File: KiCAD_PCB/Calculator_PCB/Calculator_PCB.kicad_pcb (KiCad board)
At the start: 2 copper layers, 132 x 78 mm, 110 parts, among them J1 USB_B_Micro, J2 5034801000, J3 5034801000, SW1 SW_SPST, SW10 SW_SPST, SW11 SW_SPST, SW12 SW_SPST, SW13 SW_SPST, SW14 SW_SPST, SW15 SW_SPST, SW16 SW_SPST, SW17 SW_SPST, SW18 SW_SPST, SW19 SW_SPST, SW2 SW_SPST, SW20 SW_SPST, SW21 SW_SPST, SW22 SW_SPST, SW23 SW_SPST, SW24 SW_SPST, SW25 SW_SPST, SW26 SW_SPST, SW27 SW_SPST, SW28 SW_SPST, SW29 SW_SPST, SW3 SW_SPST, SW30 SW_SPST, SW31 SW_SPST, SW32 SW_SPST, SW33 SW_SPST, SW34 SW_SPST, SW35 SW_SPST, SW36 SW_SPST, SW37 SW_SPST, SW38 SW_SPST, SW39 SW_SPST, SW4 SW_SPST, SW40 SW_SPST, SW5 SW_SPST, SW6 SW_SPST, SW7 SW_SPST, SW8 SW_SPST, SW9 SW_SPST, U1 W25Q128JVS, U2 RP2040, U3 NCP1117-3.3_SOT223, Y1 ABLS-12.000MHZ-B4-T

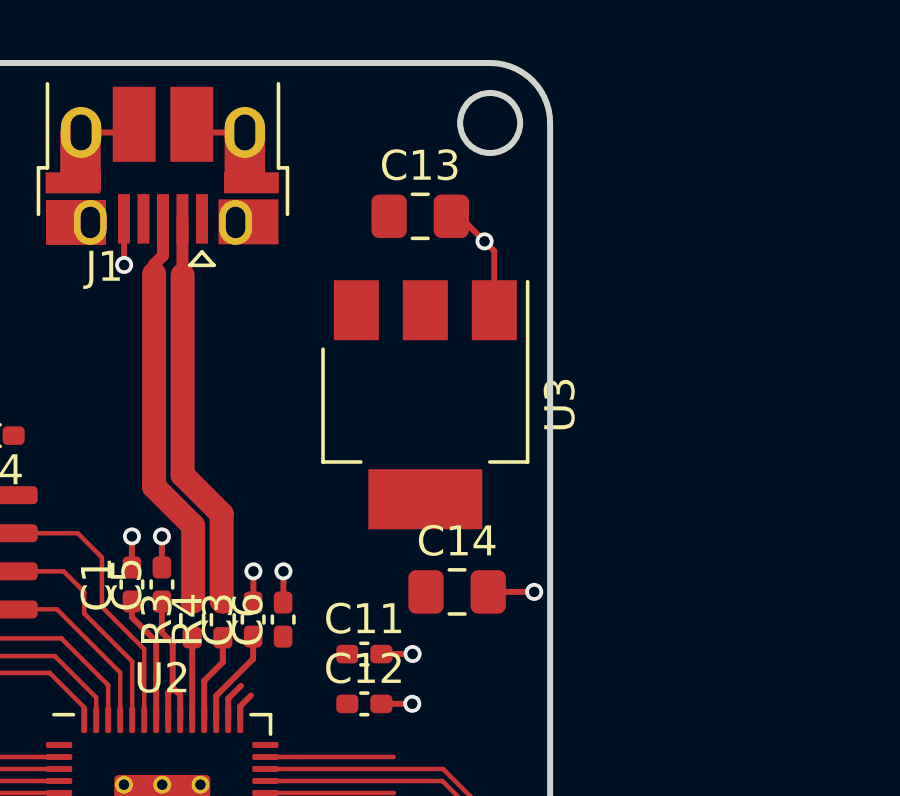
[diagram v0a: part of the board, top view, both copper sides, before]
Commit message: PCB Updates
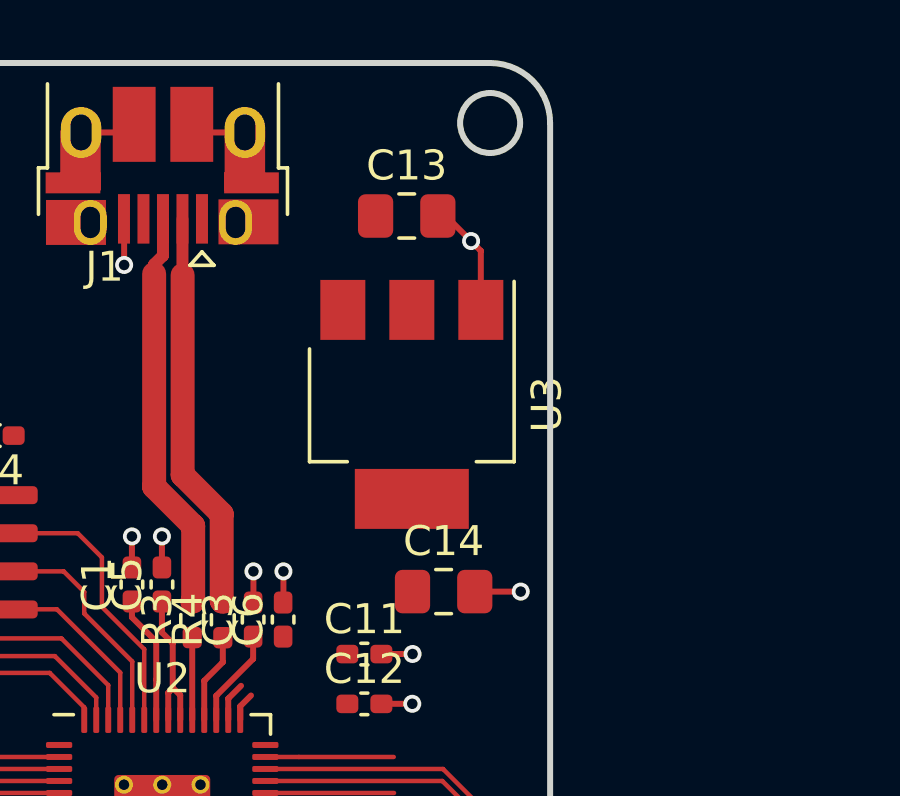
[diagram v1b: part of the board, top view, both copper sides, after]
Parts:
- moved C14 0.45 mm to (106.1, 81.8)
- moved C13 0.45 mm to (104.9, 69.3)
- moved U3 0.45 mm to (105.0, 75.6)
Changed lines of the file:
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@@
   )
   (footprint "Capacitor_SMD:C_0805_2012Metric_Pad1.18x1.45mm_HandSolder" (layer "F.Cu")
-    (at 105.32 69.32)
+    (at 104.87 69.31)
     (descr "Capacitor SMD 0805 (2012 Metric), square (rectangular) end terminal, IPC_7351 nominal with elongated pad for handsoldering. (Body size source: IPC-SM-782 page 76, https://www.pcb-3d.com/wordpress/wp-content/uploads/ipc-sm-782a_amendment_1_and_2.pdf, https://docs.google.com/spreadsheets/d/1BsfQQcO9C6DZCsRaXUlFlo91Tg2WpOkGARC1WS5S8t0/edit?usp=sharing), generated with kicad-footprint-generator")
     (tags "capacitor handsolder")
@@
   )
   (footprint "Capacitor_SMD:C_0805_2012Metric_Pad1.18x1.45mm_HandSolder" (layer "F.Cu")
-    (at 106.55 81.84)
+    (at 106.1 81.83)
     (descr "Capacitor SMD 0805 (2012 Metric), square (rectangular) end terminal, IPC_7351 nominal with elongated pad for handsoldering. (Body size source: IPC-SM-782 page 76, https://www.pcb-3d.com/wordpress/wp-content/uploads/ipc-sm-782a_amendment_1_and_2.pdf, https://docs.google.com/spreadsheets/d/1BsfQQcO9C6DZCsRaXUlFlo91Tg2WpOkGARC1WS5S8t0/edit?usp=sharing), generated with kicad-footprint-generator")
     (tags "capacitor handsolder")
@@
   )
   (footprint "Package_TO_SOT_SMD:SOT-223-3_TabPin2" (layer "F.Cu")
-    (at 105.49 75.6 -90)
+    (at 105.04 75.59 -90)
     (descr "module CMS SOT223 4 pins")
     (tags "CMS SOT")
@@
   (segment (start 95.515 66.525) (end 95.785 66.255) (width 0.2) (layer "F.Cu") (net 11))
   (segment (start 97.975 66.525) (end 97.705 66.255) (width 0.2) (layer "F.Cu") (net 11))
-  (segment (start 106.3575 69.32) (end 106.63 69.32) (width 0.2) (layer "F.Cu") (net 11))
-  (segment (start 107.5875 81.84) (end 109.12 81.84) (width 0.2) (layer "F.Cu") (net 11))
+  (segment (start 105.9075 69.31) (end 106.18 69.31) (width 0.2) (layer "F.Cu") (net 11))
+  (segment (start 107.1375 81.83) (end 108.67 81.83) (width 0.2) (layer "F.Cu") (net 11))
   (segment (start 97.005 99.21) (end 98.04 99.21) (width 0.2) (layer "F.Cu") (net 11))
-  (segment (start 106.63 69.32) (end 107.465 70.155) (width 0.2) (layer "F.Cu") (net 11))
-  (segment (start 107.465 70.155) (end 107.66 70.35) (width 0.2) (layer "F.Cu") (net 11))
+  (segment (start 106.18 69.31) (end 107.015 70.145) (width 0.2) (layer "F.Cu") (net 11))
+  (segment (start 107.015 70.145) (end 107.21 70.34) (width 0.2) (layer "F.Cu") (net 11))
   (segment (start 89.4 90.8075) (end 88.365 90.8075) (width 0.2) (layer "F.Cu") (net 11))
   (segment (start 99.76 82.19) (end 99.76 81.155) (width 0.2) (layer "F.Cu") (net 11))
   (segment (start 92.58 99.21) (end 91.545 99.21) (width 0.2) (layer "F.Cu") (net 11))
-  (segment (start 107.66 70.35) (end 107.79 70.48) (width 0.2) (layer "F.Cu") (net 11))
+  (segment (start 107.21 70.34) (end 107.34 70.47) (width 0.2) (layer "F.Cu") (net 11))
   (segment (start 95.72 92.98) (end 95.72 94.52) (width 0.2) (layer "F.Cu") (net 11))
   (segment (start 88.74 73.18) (end 88.74 74.215) (width 0.2) (layer "F.Cu") (net 11))
@@
   (segment (start 94.015 66.525) (end 95.515 66.525) (width 0.2) (layer "F.Cu") (net 11))
   (segment (start 95.45 69.41) (end 95.45 70.9425) (width 0.2) (layer "F.Cu") (net 11))
-  (segment (start 107.79 70.48) (end 107.79 72.45) (width 0.2) (layer "F.Cu") (net 11))
+  (segment (start 107.34 70.47) (end 107.34 72.44) (width 0.2) (layer "F.Cu") (net 11))
   (segment (start 104.03 90.81) (end 105.065 90.81) (width 0.2) (layer "F.Cu") (net 11))
   (segment (start 97.19 96.85) (end 97.19 97.885) (width 0.2) (layer "F.Cu") (net 11))
@@
   (via (at 105.055 85.57) (size 0.6) (drill 0.35) (layers "F.Cu" "B.Cu") (net 11))
   (via (at 105.065 83.91) (size 0.6) (drill 0.35) (layers "F.Cu" "B.Cu") (net 11))
-  (via (at 109.12 81.84) (size 0.6) (drill 0.35) (layers "F.Cu" "B.Cu") (net 11))
+  (via (at 108.67 81.83) (size 0.6) (drill 0.35) (layers "F.Cu" "B.Cu") (net 11))
   (via (at 97.19 97.885) (size 0.6) (drill 0.35) (layers "F.Cu" "B.Cu") (net 11))
   (via (at 98.04 99.21) (size 0.6) (drill 0.35) (layers "F.Cu" "B.Cu") (net 11))
@@
   (via (at 95.45 70.9425) (size 0.6) (drill 0.35) (layers "F.Cu" "B.Cu") (net 11))
   (via (at 88.74 74.215) (size 0.6) (drill 0.35) (layers "F.Cu" "B.Cu") (net 11))
-  (via (at 107.465 70.155) (size 0.6) (drill 0.35) (layers "F.Cu" "B.Cu") (net 11))
+  (via (at 107.015 70.145) (size 0.6) (drill 0.35) (layers "F.Cu" "B.Cu") (net 11))
   (segment (start 80.71 112.859616) (end 80.26243 113.307186) (width 0.15) (layer "F.Cu") (net 12))
   (segment (start 204.960864 111.83) (end 204.10952 112.681344) (width 0.15) (layer "F.Cu") (net 12))
